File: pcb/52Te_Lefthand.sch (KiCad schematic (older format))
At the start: 55 parts, among them J1 MJ-4PP-9, SW1 SW_PUSH, SW10 SW_PUSH, SW11 SW_PUSH, SW12 SW_PUSH, SW13 SW_PUSH, SW14 SW_PUSH, SW15 SW_PUSH, SW16 SW_PUSH, SW17 SW_PUSH, SW18 SW_PUSH, SW19 SW_PUSH, SW2 SW_PUSH, SW20 SW_PUSH, SW21 SW_PUSH, SW22 SW_PUSH, SW23 SW_PUSH, SW24 SW_PUSH, SW25 SW_PUSH, SW26 SW_PUSH, SW27 SW_PUSH, SW3 SW_PUSH, SW4 SW_PUSH, SW5 SW_PUSH, SW6 SW_PUSH, SW7 SW_PUSH, SW8 SW_PUSH, SW9 SW_PUSH, U1 ProMicro

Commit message: EOD 20190121 at work
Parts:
- D1, D10, D11, D12, D13, D14, D15, D16, D17, D18, D19, D2, D20, D21, D22, D23, D24, D25, D26, D3, D4, D5, D6, D7, D8, D9: footprint (none) -> kbd:D3_SMD
- J1: footprint (none) -> kbd:MJ-4PP-9

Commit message: 20190122 placement
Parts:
- SW1, SW10, SW11, SW12, SW13, SW14, SW15, SW16, SW17, SW18, SW19, SW2, SW20, SW21, SW22, SW23, SW24, SW25, SW26, SW3, SW4, SW5, SW6, SW7, SW8, SW9: footprint (none) -> Kailh:CPG151101S11
- SW27: footprint (none) -> kbd:ResetSW
- U1: footprint (none) -> kbd:ProMicro_v2_FaceDown
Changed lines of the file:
@@
 F 0 "U1" H 9150 4587 60  0000 C CNN
 F 1 "ProMicro" H 9150 4481 60  0000 C CNN
-F 2 "" H 9250 2500 60  0001 C CNN
+F 2 "kbd:ProMicro_v2_FaceDown" H 9250 2500 60  0001 C CNN
 F 3 "" H 9250 2500 60  0000 C CNN
 	1    9150 3550
@@
 F 0 "SW27" H 9200 4655 50  0000 C CNN
 F 1 "SW_PUSH" H 9200 4564 50  0000 C CNN
-F 2 "" H 9200 4400 50  0001 C CNN
+F 2 "kbd:ResetSW" H 9200 4400 50  0001 C CNN
 F 3 "" H 9200 4400 50  0000 C CNN
 	1    9200 4400
@@
 F 0 "SW1" H 1500 3555 50  0000 C CNN
 F 1 "SW_PUSH" H 1500 3464 50  0000 C CNN
-F 2 "" H 1500 3300 50  0001 C CNN
+F 2 "Kailh:CPG151101S11" H 1500 3300 50  0001 C CNN
 F 3 "" H 1500 3300 50  0000 C CNN
 	1    1500 3300
@@
 F 0 "SW2" H 1500 4255 50  0000 C CNN
 F 1 "SW_PUSH" H 1500 4164 50  0000 C CNN
-F 2 "" H 1500 4000 50  0001 C CNN
+F 2 "Kailh:CPG151101S11" H 1500 4000 50  0001 C CNN
 F 3 "" H 1500 4000 50  0000 C CNN
 	1    1500 4000
@@
 F 0 "SW3" H 1500 4955 50  0000 C CNN
 F 1 "SW_PUSH" H 1500 4864 50  0000 C CNN
-F 2 "" H 1500 4700 50  0001 C CNN
+F 2 "Kailh:CPG151101S11" H 1500 4700 50  0001 C CNN
 F 3 "" H 1500 4700 50  0000 C CNN
 	1    1500 4700
@@
 F 0 "SW5" H 2500 3555 50  0000 C CNN
 F 1 "SW_PUSH" H 2500 3464 50  0000 C CNN
-F 2 "" H 2500 3300 50  0001 C CNN
+F 2 "Kailh:CPG151101S11" H 2500 3300 50  0001 C CNN
 F 3 "" H 2500 3300 50  0000 C CNN
 	1    2500 3300
@@
 F 0 "SW6" H 2500 4255 50  0000 C CNN
 F 1 "SW_PUSH" H 2500 4164 50  0000 C CNN
-F 2 "" H 2500 4000 50  0001 C CNN
+F 2 "Kailh:CPG151101S11" H 2500 4000 50  0001 C CNN
 F 3 "" H 2500 4000 50  0000 C CNN
 	1    2500 4000
@@
 F 0 "SW7" H 2500 4955 50  0000 C CNN
 F 1 "SW_PUSH" H 2500 4864 50  0000 C CNN
-F 2 "" H 2500 4700 50  0001 C CNN
+F 2 "Kailh:CPG151101S11" H 2500 4700 50  0001 C CNN
 F 3 "" H 2500 4700 50  0000 C CNN
 	1    2500 4700
@@
 F 0 "SW9" H 3500 3555 50  0000 C CNN
 F 1 "SW_PUSH" H 3500 3464 50  0000 C CNN
-F 2 "" H 3500 3300 50  0001 C CNN
+F 2 "Kailh:CPG151101S11" H 3500 3300 50  0001 C CNN
 F 3 "" H 3500 3300 50  0000 C CNN
 	1    3500 3300
@@
 F 0 "SW10" H 3500 4255 50  0000 C CNN
 F 1 "SW_PUSH" H 3500 4164 50  0000 C CNN
-F 2 "" H 3500 4000 50  0001 C CNN
+F 2 "Kailh:CPG151101S11" H 3500 4000 50  0001 C CNN
 F 3 "" H 3500 4000 50  0000 C CNN
 	1    3500 4000
@@
 F 0 "SW11" H 3500 4955 50  0000 C CNN
 F 1 "SW_PUSH" H 3500 4864 50  0000 C CNN
-F 2 "" H 3500 4700 50  0001 C CNN
+F 2 "Kailh:CPG151101S11" H 3500 4700 50  0001 C CNN
 F 3 "" H 3500 4700 50  0000 C CNN
 	1    3500 4700
@@
 F 0 "SW13" H 4500 3555 50  0000 C CNN
 F 1 "SW_PUSH" H 4500 3464 50  0000 C CNN
-F 2 "" H 4500 3300 50  0001 C CNN
+F 2 "Kailh:CPG151101S11" H 4500 3300 50  0001 C CNN
 F 3 "" H 4500 3300 50  0000 C CNN
 	1    4500 3300
@@
 F 0 "SW14" H 4500 4255 50  0000 C CNN
 F 1 "SW_PUSH" H 4500 4164 50  0000 C CNN
-F 2 "" H 4500 4000 50  0001 C CNN
+F 2 "Kailh:CPG151101S11" H 4500 4000 50  0001 C CNN
 F 3 "" H 4500 4000 50  0000 C CNN
 	1    4500 4000
@@
 F 0 "SW15" H 4500 4955 50  0000 C CNN
 F 1 "SW_PUSH" H 4500 4864 50  0000 C CNN
-F 2 "" H 4500 4700 50  0001 C CNN
+F 2 "Kailh:CPG151101S11" H 4500 4700 50  0001 C CNN
 F 3 "" H 4500 4700 50  0000 C CNN
 	1    4500 4700
@@
 F 0 "SW18" H 5500 3555 50  0000 C CNN
 F 1 "SW_PUSH" H 5500 3464 50  0000 C CNN
-F 2 "" H 5500 3300 50  0001 C CNN
+F 2 "Kailh:CPG151101S11" H 5500 3300 50  0001 C CNN
 F 3 "" H 5500 3300 50  0000 C CNN
 	1    5500 3300
@@
 F 0 "SW19" H 5500 4255 50  0000 C CNN
 F 1 "SW_PUSH" H 5500 4164 50  0000 C CNN
-F 2 "" H 5500 4000 50  0001 C CNN
+F 2 "Kailh:CPG151101S11" H 5500 4000 50  0001 C CNN
 F 3 "" H 5500 4000 50  0000 C CNN
 	1    5500 4000
@@
 F 0 "SW20" H 5500 4955 50  0000 C CNN
 F 1 "SW_PUSH" H 5500 4864 50  0000 C CNN
-F 2 "" H 5500 4700 50  0001 C CNN
+F 2 "Kailh:CPG151101S11" H 5500 4700 50  0001 C CNN
 F 3 "" H 5500 4700 50  0000 C CNN
 	1    5500 4700
@@
 F 0 "SW23" H 6500 3555 50  0000 C CNN
 F 1 "SW_PUSH" H 6500 3464 50  0000 C CNN
-F 2 "" H 6500 3300 50  0001 C CNN
+F 2 "Kailh:CPG151101S11" H 6500 3300 50  0001 C CNN
 F 3 "" H 6500 3300 50  0000 C CNN
 	1    6500 3300
@@
 F 0 "SW24" H 6500 4255 50  0000 C CNN
 F 1 "SW_PUSH" H 6500 4164 50  0000 C CNN
-F 2 "" H 6500 4000 50  0001 C CNN
+F 2 "Kailh:CPG151101S11" H 6500 4000 50  0001 C CNN
 F 3 "" H 6500 4000 50  0000 C CNN
 	1    6500 4000
@@
 F 0 "SW25" H 6500 4955 50  0000 C CNN
 F 1 "SW_PUSH" H 6500 4864 50  0000 C CNN
-F 2 "" H 6500 4700 50  0001 C CNN
+F 2 "Kailh:CPG151101S11" H 6500 4700 50  0001 C CNN
 F 3 "" H 6500 4700 50  0000 C CNN
 	1    6500 4700
@@
 F 0 "SW4" H 2500 2855 50  0000 C CNN
 F 1 "SW_PUSH" H 2500 2764 50  0000 C CNN
-F 2 "" H 2500 2600 50  0001 C CNN
+F 2 "Kailh:CPG151101S11" H 2500 2600 50  0001 C CNN
 F 3 "" H 2500 2600 50  0000 C CNN
 	1    2500 2600
@@
 F 0 "SW8" H 3500 2855 50  0000 C CNN
 F 1 "SW_PUSH" H 3500 2764 50  0000 C CNN
-F 2 "" H 3500 2600 50  0001 C CNN
+F 2 "Kailh:CPG151101S11" H 3500 2600 50  0001 C CNN
 F 3 "" H 3500 2600 50  0000 C CNN
 	1    3500 2600
@@
 F 0 "SW12" H 4500 2855 50  0000 C CNN
 F 1 "SW_PUSH" H 4500 2764 50  0000 C CNN
-F 2 "" H 4500 2600 50  0001 C CNN
+F 2 "Kailh:CPG151101S11" H 4500 2600 50  0001 C CNN
 F 3 "" H 4500 2600 50  0000 C CNN
 	1    4500 2600
@@
 F 0 "SW17" H 5500 2855 50  0000 C CNN
 F 1 "SW_PUSH" H 5500 2764 50  0000 C CNN
-F 2 "" H 5500 2600 50  0001 C CNN
+F 2 "Kailh:CPG151101S11" H 5500 2600 50  0001 C CNN
 F 3 "" H 5500 2600 50  0000 C CNN
 	1    5500 2600
@@
 F 0 "SW22" H 6500 2855 50  0000 C CNN
 F 1 "SW_PUSH" H 6500 2764 50  0000 C CNN
-F 2 "" H 6500 2600 50  0001 C CNN
+F 2 "Kailh:CPG151101S11" H 6500 2600 50  0001 C CNN
 F 3 "" H 6500 2600 50  0000 C CNN
 	1    6500 2600
@@
 F 0 "SW16" H 4500 5655 50  0000 C CNN
 F 1 "SW_PUSH" H 4500 5564 50  0000 C CNN
-F 2 "" H 4500 5400 50  0001 C CNN
+F 2 "Kailh:CPG151101S11" H 4500 5400 50  0001 C CNN
 F 3 "" H 4500 5400 50  0000 C CNN
 	1    4500 5400
@@
 F 0 "SW21" H 5500 5655 50  0000 C CNN
 F 1 "SW_PUSH" H 5500 5564 50  0000 C CNN
-F 2 "" H 5500 5400 50  0001 C CNN
+F 2 "Kailh:CPG151101S11" H 5500 5400 50  0001 C CNN
 F 3 "" H 5500 5400 50  0000 C CNN
 	1    5500 5400
@@
 F 0 "SW26" H 6500 5655 50  0000 C CNN
 F 1 "SW_PUSH" H 6500 5564 50  0000 C CNN
-F 2 "" H 6500 5400 50  0001 C CNN
+F 2 "Kailh:CPG151101S11" H 6500 5400 50  0001 C CNN
 F 3 "" H 6500 5400 50  0000 C CNN
 	1    6500 5400

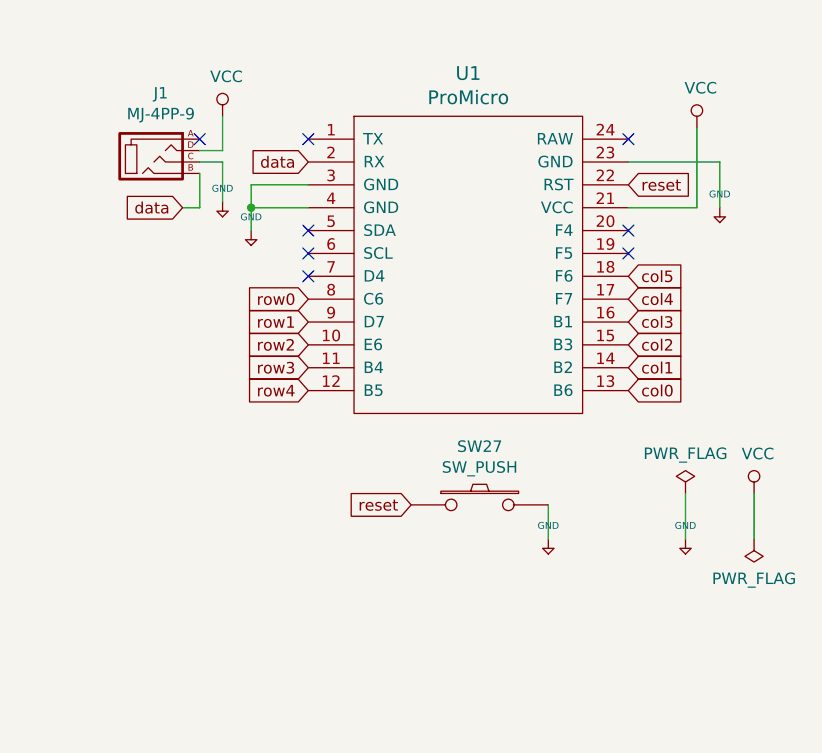
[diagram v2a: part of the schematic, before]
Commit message: first draft pcb lefthand
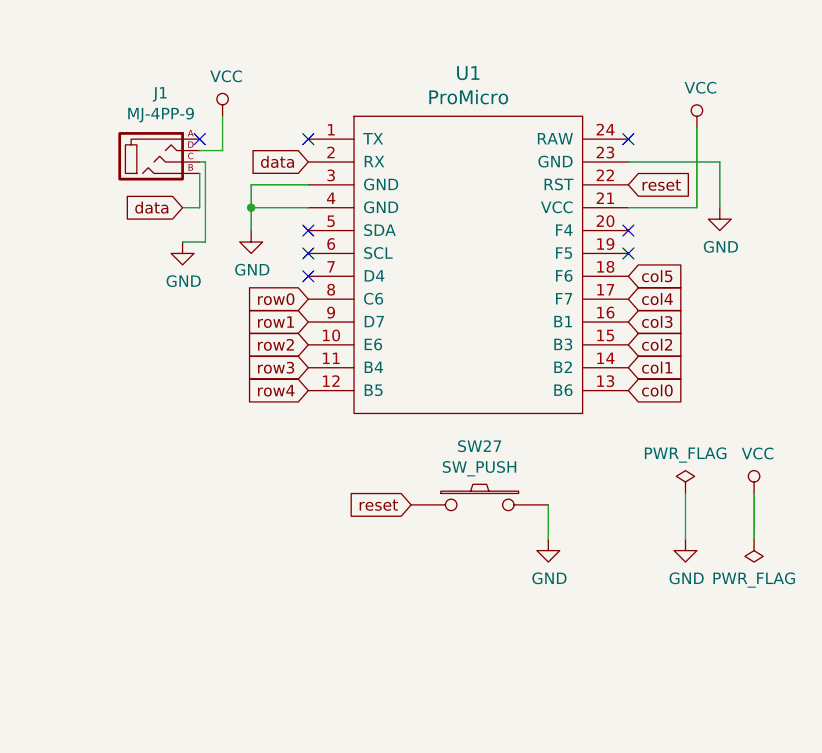
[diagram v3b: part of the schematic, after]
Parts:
- D1, D10, D11, D12, D13, D14, D15, D16, D17, D18, D19, D2, D20, D21, D22, D23, D24, D25, D26, D3, D4, D5, D6, D7, D8, D9: footprint kbd:D3_SMD -> Diode_SMD:D_SOD-123
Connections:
- net +5V renamed GND
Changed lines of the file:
@@
-$EndComp
-$Comp
-L keyboard_parts:GND #PWR0101
-U 1 1 5C491A1C
-P 10250 3100
-F 0 "#PWR0101" H 10250 3150 20  0001 C CNN
-F 1 "GND" H 10250 3159 30  0000 C CNN
-F 2 "" H 10250 3100 60  0000 C CNN
-F 3 "" H 10250 3100 60  0000 C CNN
-	1    10250 3100
-	1    0    0    -1
-$EndComp
-$Comp
-L keyboard_parts:GND #PWR0102
-U 1 1 5C491A53
-P 8200 3200
-F 0 "#PWR0102" H 8200 3250 20  0001 C CNN
-F 1 "GND" H 8200 3259 30  0000 C CNN
-F 2 "" H 8200 3200 60  0000 C CNN
-F 3 "" H 8200 3200 60  0000 C CNN
-	1    8200 3200
-	1    0    0    -1
 $EndComp
 $Comp
@@
 	1    0    0    -1
 $EndComp
-$Comp
-L keyboard_parts:GND #PWR0104
-U 1 1 5C491BA4
-P 9500 4550
-F 0 "#PWR0104" H 9500 4600 20  0001 C CNN
-F 1 "GND" H 9500 4609 30  0000 C CNN
-F 2 "" H 9500 4550 60  0000 C CNN
-F 3 "" H 9500 4550 60  0000 C CNN
-	1    9500 4550
-	1    0    0    -1
-$EndComp
 Wire Wire Line
 	9500 4400 9500 4550
@@
 $EndComp
 NoConn ~ 7975 2800
-$Comp
-L keyboard_parts:GND #PWR0105
-U 1 1 5C491E36
-P 8075 3075
-F 0 "#PWR0105" H 8075 3125 20  0001 C CNN
-F 1 "GND" H 8075 3134 30  0000 C CNN
-F 2 "" H 8075 3075 60  0000 C CNN
-F 3 "" H 8075 3075 60  0000 C CNN
-	1    8075 3075
-	1    0    0    -1
-$EndComp
-Wire Wire Line
-	7975 2900 8075 2900
-Wire Wire Line
-	8075 2900 8075 3075
+Wire Wire Line
+	7975 2900 8000 2900
 $Comp
 L power:VCC #PWR0106
@@
 F 0 "D4" H 2600 3016 50  0000 C CNN
 F 1 "D" H 2600 2925 50  0000 C CNN
-F 2 "kbd:D3_SMD" H 2600 2800 50  0001 C CNN
+F 2 "Diode_SMD:D_SOD-123" H 2600 2800 50  0001 C CNN
 F 3 "~" H 2600 2800 50  0001 C CNN
 	1    2600 2800
@@
 F 0 "D8" H 3600 3016 50  0000 C CNN
 F 1 "D" H 3600 2925 50  0000 C CNN
-F 2 "kbd:D3_SMD" H 3600 2800 50  0001 C CNN
+F 2 "Diode_SMD:D_SOD-123" H 3600 2800 50  0001 C CNN
 F 3 "~" H 3600 2800 50  0001 C CNN
 	1    3600 2800
@@
 F 0 "D12" H 4600 3016 50  0000 C CNN
 F 1 "D" H 4600 2925 50  0000 C CNN
-F 2 "kbd:D3_SMD" H 4600 2800 50  0001 C CNN
+F 2 "Diode_SMD:D_SOD-123" H 4600 2800 50  0001 C CNN
 F 3 "~" H 4600 2800 50  0001 C CNN
 	1    4600 2800
@@
 F 0 "D17" H 5600 3016 50  0000 C CNN
 F 1 "D" H 5600 2925 50  0000 C CNN
-F 2 "kbd:D3_SMD" H 5600 2800 50  0001 C CNN
+F 2 "Diode_SMD:D_SOD-123" H 5600 2800 50  0001 C CNN
 F 3 "~" H 5600 2800 50  0001 C CNN
 	1    5600 2800
@@
 F 0 "D22" H 6600 3016 50  0000 C CNN
 F 1 "D" H 6600 2925 50  0000 C CNN
-F 2 "kbd:D3_SMD" H 6600 2800 50  0001 C CNN
+F 2 "Diode_SMD:D_SOD-123" H 6600 2800 50  0001 C CNN
 F 3 "~" H 6600 2800 50  0001 C CNN
 	1    6600 2800
@@
 F 0 "D5" H 2600 3716 50  0000 C CNN
 F 1 "D" H 2600 3625 50  0000 C CNN
-F 2 "kbd:D3_SMD" H 2600 3500 50  0001 C CNN
+F 2 "Diode_SMD:D_SOD-123" H 2600 3500 50  0001 C CNN
 F 3 "~" H 2600 3500 50  0001 C CNN
 	1    2600 3500
@@
 F 0 "D9" H 3600 3716 50  0000 C CNN
 F 1 "D" H 3600 3625 50  0000 C CNN
-F 2 "kbd:D3_SMD" H 3600 3500 50  0001 C CNN
+F 2 "Diode_SMD:D_SOD-123" H 3600 3500 50  0001 C CNN
 F 3 "~" H 3600 3500 50  0001 C CNN
 	1    3600 3500
@@
 F 0 "D13" H 4600 3716 50  0000 C CNN
 F 1 "D" H 4600 3625 50  0000 C CNN
-F 2 "kbd:D3_SMD" H 4600 3500 50  0001 C CNN
+F 2 "Diode_SMD:D_SOD-123" H 4600 3500 50  0001 C CNN
 F 3 "~" H 4600 3500 50  0001 C CNN
 	1    4600 3500
@@
 F 0 "D18" H 5600 3716 50  0000 C CNN
 F 1 "D" H 5600 3625 50  0000 C CNN
-F 2 "kbd:D3_SMD" H 5600 3500 50  0001 C CNN
+F 2 "Diode_SMD:D_SOD-123" H 5600 3500 50  0001 C CNN
 F 3 "~" H 5600 3500 50  0001 C CNN
 	1    5600 3500
@@
 F 0 "D23" H 6600 3716 50  0000 C CNN
 F 1 "D" H 6600 3625 50  0000 C CNN
-F 2 "kbd:D3_SMD" H 6600 3500 50  0001 C CNN
+F 2 "Diode_SMD:D_SOD-123" H 6600 3500 50  0001 C CNN
 F 3 "~" H 6600 3500 50  0001 C CNN
 	1    6600 3500
@@
 F 0 "D6" H 2600 4416 50  0000 C CNN
 F 1 "D" H 2600 4325 50  0000 C CNN
-F 2 "kbd:D3_SMD" H 2600 4200 50  0001 C CNN
+F 2 "Diode_SMD:D_SOD-123" H 2600 4200 50  0001 C CNN
 F 3 "~" H 2600 4200 50  0001 C CNN
 	1    2600 4200
@@
 F 0 "D10" H 3600 4416 50  0000 C CNN
 F 1 "D" H 3600 4325 50  0000 C CNN
-F 2 "kbd:D3_SMD" H 3600 4200 50  0001 C CNN
+F 2 "Diode_SMD:D_SOD-123" H 3600 4200 50  0001 C CNN
 F 3 "~" H 3600 4200 50  0001 C CNN
 	1    3600 4200
@@
 F 0 "D14" H 4600 4416 50  0000 C CNN
 F 1 "D" H 4600 4325 50  0000 C CNN
-F 2 "kbd:D3_SMD" H 4600 4200 50  0001 C CNN
+F 2 "Diode_SMD:D_SOD-123" H 4600 4200 50  0001 C CNN
 F 3 "~" H 4600 4200 50  0001 C CNN
 	1    4600 4200
@@
 F 0 "D19" H 5600 4416 50  0000 C CNN
 F 1 "D" H 5600 4325 50  0000 C CNN
-F 2 "kbd:D3_SMD" H 5600 4200 50  0001 C CNN
+F 2 "Diode_SMD:D_SOD-123" H 5600 4200 50  0001 C CNN
 F 3 "~" H 5600 4200 50  0001 C CNN
 	1    5600 4200
@@
 F 0 "D24" H 6600 4416 50  0000 C CNN
 F 1 "D" H 6600 4325 50  0000 C CNN
-F 2 "kbd:D3_SMD" H 6600 4200 50  0001 C CNN
+F 2 "Diode_SMD:D_SOD-123" H 6600 4200 50  0001 C CNN
 F 3 "~" H 6600 4200 50  0001 C CNN
 	1    6600 4200
@@
 F 0 "D7" H 2600 5116 50  0000 C CNN
 F 1 "D" H 2600 5025 50  0000 C CNN
-F 2 "kbd:D3_SMD" H 2600 4900 50  0001 C CNN
+F 2 "Diode_SMD:D_SOD-123" H 2600 4900 50  0001 C CNN
 F 3 "~" H 2600 4900 50  0001 C CNN
 	1    2600 4900
@@
 F 0 "D11" H 3600 5116 50  0000 C CNN
 F 1 "D" H 3600 5025 50  0000 C CNN
-F 2 "kbd:D3_SMD" H 3600 4900 50  0001 C CNN
+F 2 "Diode_SMD:D_SOD-123" H 3600 4900 50  0001 C CNN
 F 3 "~" H 3600 4900 50  0001 C CNN
 	1    3600 4900
@@
 F 0 "D15" H 4600 5116 50  0000 C CNN
 F 1 "D" H 4600 5025 50  0000 C CNN
-F 2 "kbd:D3_SMD" H 4600 4900 50  0001 C CNN
+F 2 "Diode_SMD:D_SOD-123" H 4600 4900 50  0001 C CNN
 F 3 "~" H 4600 4900 50  0001 C CNN
 	1    4600 4900
@@
 F 0 "D20" H 5600 5116 50  0000 C CNN
 F 1 "D" H 5600 5025 50  0000 C CNN
-F 2 "kbd:D3_SMD" H 5600 4900 50  0001 C CNN
+F 2 "Diode_SMD:D_SOD-123" H 5600 4900 50  0001 C CNN
 F 3 "~" H 5600 4900 50  0001 C CNN
 	1    5600 4900
@@
 F 0 "D25" H 6600 5116 50  0000 C CNN
 F 1 "D" H 6600 5025 50  0000 C CNN
-F 2 "kbd:D3_SMD" H 6600 4900 50  0001 C CNN
+F 2 "Diode_SMD:D_SOD-123" H 6600 4900 50  0001 C CNN
 F 3 "~" H 6600 4900 50  0001 C CNN
 	1    6600 4900
@@
 F 0 "D1" H 1600 3716 50  0000 C CNN
 F 1 "D" H 1600 3625 50  0000 C CNN
-F 2 "kbd:D3_SMD" H 1600 3500 50  0001 C CNN
+F 2 "Diode_SMD:D_SOD-123" H 1600 3500 50  0001 C CNN
 F 3 "~" H 1600 3500 50  0001 C CNN
 	1    1600 3500
@@
 F 0 "D2" H 1600 4416 50  0000 C CNN
 F 1 "D" H 1600 4325 50  0000 C CNN
-F 2 "kbd:D3_SMD" H 1600 4200 50  0001 C CNN
+F 2 "Diode_SMD:D_SOD-123" H 1600 4200 50  0001 C CNN
 F 3 "~" H 1600 4200 50  0001 C CNN
 	1    1600 4200
@@
 F 0 "D3" H 1600 5116 50  0000 C CNN
 F 1 "D" H 1600 5025 50  0000 C CNN
-F 2 "kbd:D3_SMD" H 1600 4900 50  0001 C CNN
+F 2 "Diode_SMD:D_SOD-123" H 1600 4900 50  0001 C CNN
 F 3 "~" H 1600 4900 50  0001 C CNN
 	1    1600 4900
@@
 F 0 "D16" H 4600 5816 50  0000 C CNN
 F 1 "D" H 4600 5725 50  0000 C CNN
-F 2 "kbd:D3_SMD" H 4600 5600 50  0001 C CNN
+F 2 "Diode_SMD:D_SOD-123" H 4600 5600 50  0001 C CNN
 F 3 "~" H 4600 5600 50  0001 C CNN
 	1    4600 5600
@@
 F 0 "D21" H 5600 5816 50  0000 C CNN
 F 1 "D" H 5600 5725 50  0000 C CNN
-F 2 "kbd:D3_SMD" H 5600 5600 50  0001 C CNN
+F 2 "Diode_SMD:D_SOD-123" H 5600 5600 50  0001 C CNN
 F 3 "~" H 5600 5600 50  0001 C CNN
 	1    5600 5600
@@
 F 0 "D26" H 6600 5816 50  0000 C CNN
 F 1 "D" H 6600 5725 50  0000 C CNN
-F 2 "kbd:D3_SMD" H 6600 5600 50  0001 C CNN
+F 2 "Diode_SMD:D_SOD-123" H 6600 5600 50  0001 C CNN
 F 3 "~" H 6600 5600 50  0001 C CNN
 	1    6600 5600
@@
 	1    0    0    -1
 $EndComp
-$Comp
-L keyboard_parts:GND #PWR0108
-U 1 1 5C5C08D8
-P 10100 4550
-F 0 "#PWR0108" H 10100 4600 20  0001 C CNN
-F 1 "GND" H 10100 4609 30  0000 C CNN
-F 2 "" H 10100 4550 60  0000 C CNN
-F 3 "" H 10100 4550 60  0000 C CNN
-	1    10100 4550
-	1    0    0    -1
-$EndComp
 Wire Wire Line
 	10100 4350 10100 4550
@@
 NoConn ~ 9850 3300
 NoConn ~ 8450 2800
+$Comp
+L power:GND #PWR?
+U 1 1 5C484FA5
+P 7900 3250
+F 0 "#PWR?" H 7900 3000 50  0001 C CNN
+F 1 "GND" H 7905 3077 50  0000 C CNN
+F 2 "" H 7900 3250 50  0001 C CNN
+F 3 "" H 7900 3250 50  0001 C CNN
+	1    7900 3250
+	1    0    0    -1
+$EndComp
+$Comp
+L power:GND #PWR?
+U 1 1 5C49DECF
+P 8200 3200
+F 0 "#PWR?" H 8200 2950 50  0001 C CNN
+F 1 "GND" H 8205 3027 50  0000 C CNN
+F 2 "" H 8200 3200 50  0001 C CNN
+F 3 "" H 8200 3200 50  0001 C CNN
+	1    8200 3200
+	1    0    0    -1
+$EndComp
+Wire Wire Line
+	8000 2900 8000 3250
+Wire Wire Line
+	8000 3250 7900 3250
+$Comp
+L power:GND #PWR?
+U 1 1 5C4BFF4E
+P 10250 3100
+F 0 "#PWR?" H 10250 2850 50  0001 C CNN
+F 1 "GND" H 10255 2927 50  0000 C CNN
+F 2 "" H 10250 3100 50  0001 C CNN
+F 3 "" H 10250 3100 50  0001 C CNN
+	1    10250 3100
+	1    0    0    -1
+$EndComp
+$Comp
+L power:GND #PWR?
+U 1 1 5C4C851D
+P 10100 4550
+F 0 "#PWR?" H 10100 4300 50  0001 C CNN
+F 1 "GND" H 10105 4377 50  0000 C CNN
+F 2 "" H 10100 4550 50  0001 C CNN
+F 3 "" H 10100 4550 50  0001 C CNN
+	1    10100 4550
+	1    0    0    -1
+$EndComp
+$Comp
+L power:GND #PWR?
+U 1 1 5C4D0A4E
+P 9500 4550
+F 0 "#PWR?" H 9500 4300 50  0001 C CNN
+F 1 "GND" H 9505 4377 50  0000 C CNN
+F 2 "" H 9500 4550 50  0001 C CNN
+F 3 "" H 9500 4550 50  0001 C CNN
+	1    9500 4550
+	1    0    0    -1
+$EndComp
 $EndSCHEMATC
